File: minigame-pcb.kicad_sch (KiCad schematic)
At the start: 103 parts, among them IC1 HT16K33A-28SSOP, J1 USB_C_Receptacle_USB2.0_16P, U2 AMS1117-3.3, U3 W25Q128JVS, U4 RP2040, Y1 ABM8-272-T3

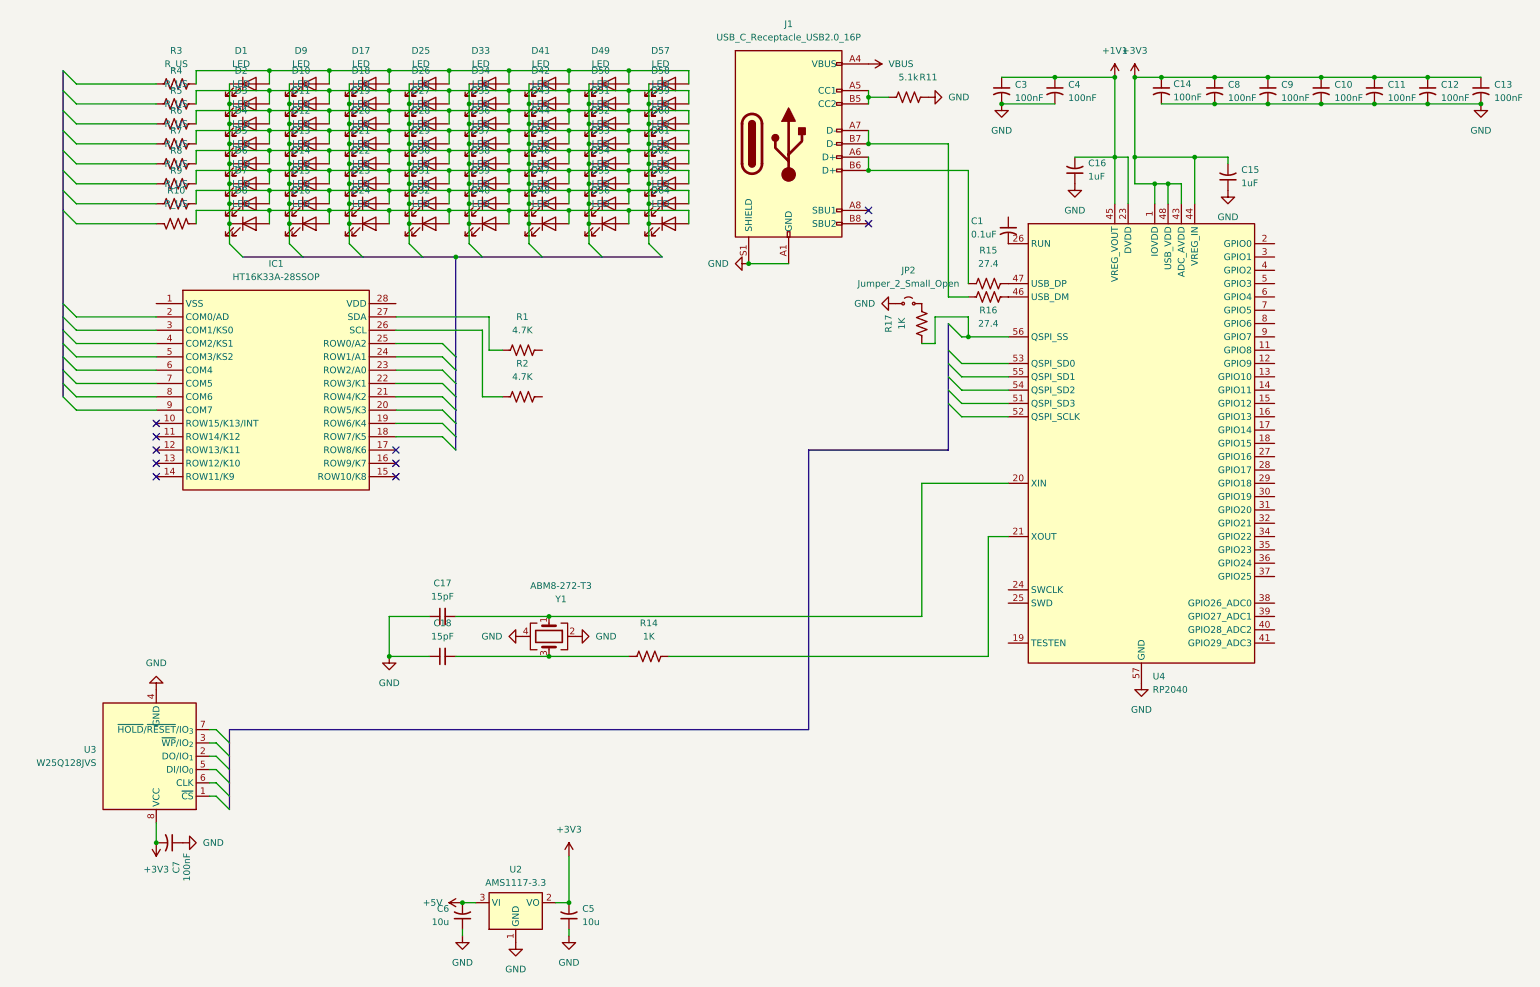
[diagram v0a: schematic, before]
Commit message: e
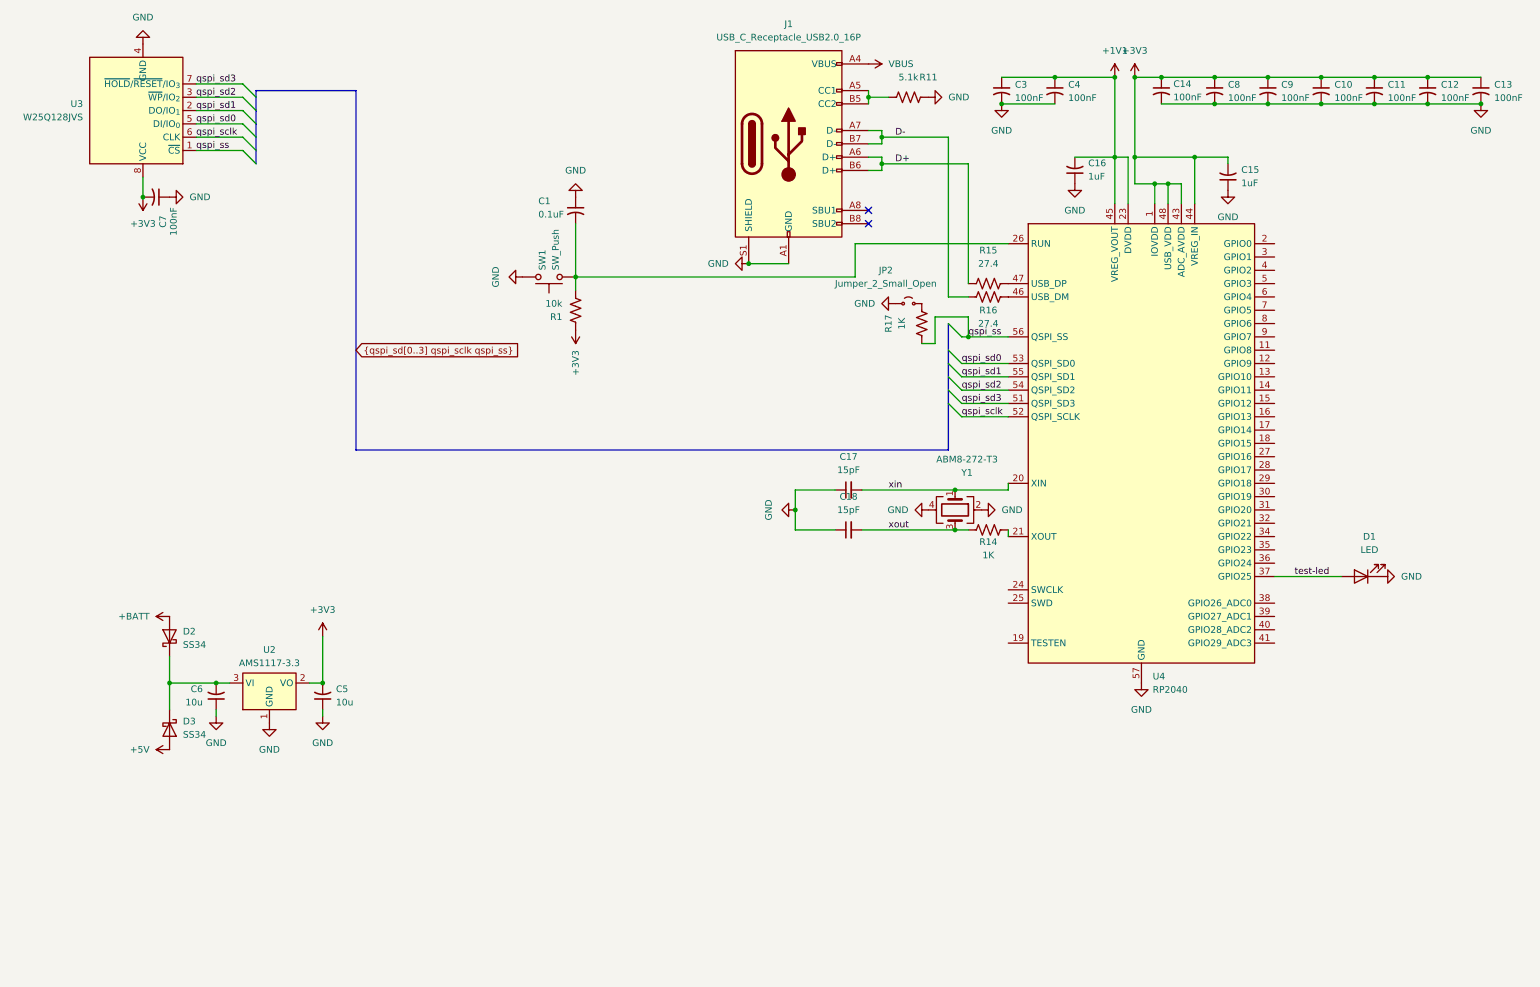
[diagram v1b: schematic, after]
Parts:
- removed D10, D11, D12, D13, D14, D15, D16, D17, D18, D19, D2, D20, D21, D22, D23, D24, D25, D26, D27, D28, D29, D3, D30, D31, D32, D33, D34, D35, D36, D37, D38, D39, D4, D40, D41, D42, D43, D44, D45, D46, D47, D48, D49, D5, D50, D51, D52, D53, D54, D55, D56, D57, D58, D59, D6, D60, D61, D62, D63, D64, D7, D8, D9: LED, LED_SMD:LED_0603_1608Metric_Pad1.05x0.95mm_HandSolder, symbol Device:LED
- removed IC1: HT16K33A-28SSOP, HT16K33A:SOP64P600X175-28N, symbol HT16K33A:HT16K33A-28SSOP
- removed R10, R3, R4, R5, R6, R7, R8, R9: R_US, symbol Device:R_US
- removed R2: 4.7K, Resistor_SMD:R_0603_1608Metric_Pad0.98x0.95mm_HandSolder, symbol Device:R_US
- added D2, D3: SS34, Diode_SMD:D_SMA, symbol Diode:SS34
- added SW1: SW_Push, symbol Switch:SW_Push
- R1: value 4.7K -> 10k
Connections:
- net +3V3: now also R1.2
- net +5V: now also D3.2 (A); no longer C6.2, U2.3 (VI)
- net GND: now also C1.1, D1.1 (K), SW1.2
- net test-led: now reaches D1.2 (A)
- net test-led: now also U4.37 (GPIO25)
- net at R1.1: now also C1.2, U4.26 (RUN), SW1.1
- net qspi_ss: now reaches U3.1 (~{CS})
- net qspi_ss: now also R17.1, U4.56 (QSPI_SS)
- net qspi_sd1: now reaches U3.2 (DO/IO_{1})
- net qspi_sd1: now also U4.55 (QSPI_SD1)
- net qspi_sd2: now reaches U3.3 (~{WP}/IO_{2})
- net qspi_sd2: now also U4.54 (QSPI_SD2)
- net qspi_sd0: now reaches U3.5 (DI/IO_{0})
- net qspi_sd0: now also U4.53 (QSPI_SD0)
- net qspi_sclk: now reaches U3.6 (CLK)
- net qspi_sclk: now also U4.52 (QSPI_SCLK)
- net qspi_sd3: now reaches U3.7 (~{HOLD}/~{RESET}/IO_{3})
- net qspi_sd3: now also U4.51 (QSPI_SD3)
- net xout: now reaches C18.2, R14.1, Y1.3
- net xin: now reaches C17.2, U4.20 (XIN), Y1.1
- net D-: now reaches J1.A7 (D-), J1.B7 (D-), R16.1
- net D+: now reaches J1.A6 (D+), J1.B6 (D+), R15.1
- new net: C6.2, D2.1 (K), D3.1 (K), U2.3 (VI)
- new net +BATT: D2.2 (A)
- no-connect marks 10 -> 2
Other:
- moved on the sheet: C1, C17, C18, C5, C6, C7, R14, U2, U3, Y1
